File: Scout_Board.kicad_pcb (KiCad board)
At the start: 2 copper layers, 102.5 x 80 mm, 57 parts, among them J1 Conn_01x01_Pin, J2 Conn_01x04_Pin, J3 RAPC722X, J4 Screw_Terminal_01x02, J5 5V, J6 GND, Q1 BSS138, Q2 BSS138, U1 DRV8871DDA, U2 ESP32-S3-DEVKITC-1U-N8R2, U3 LM2576HVS-5, U4 LM2576HVS-5

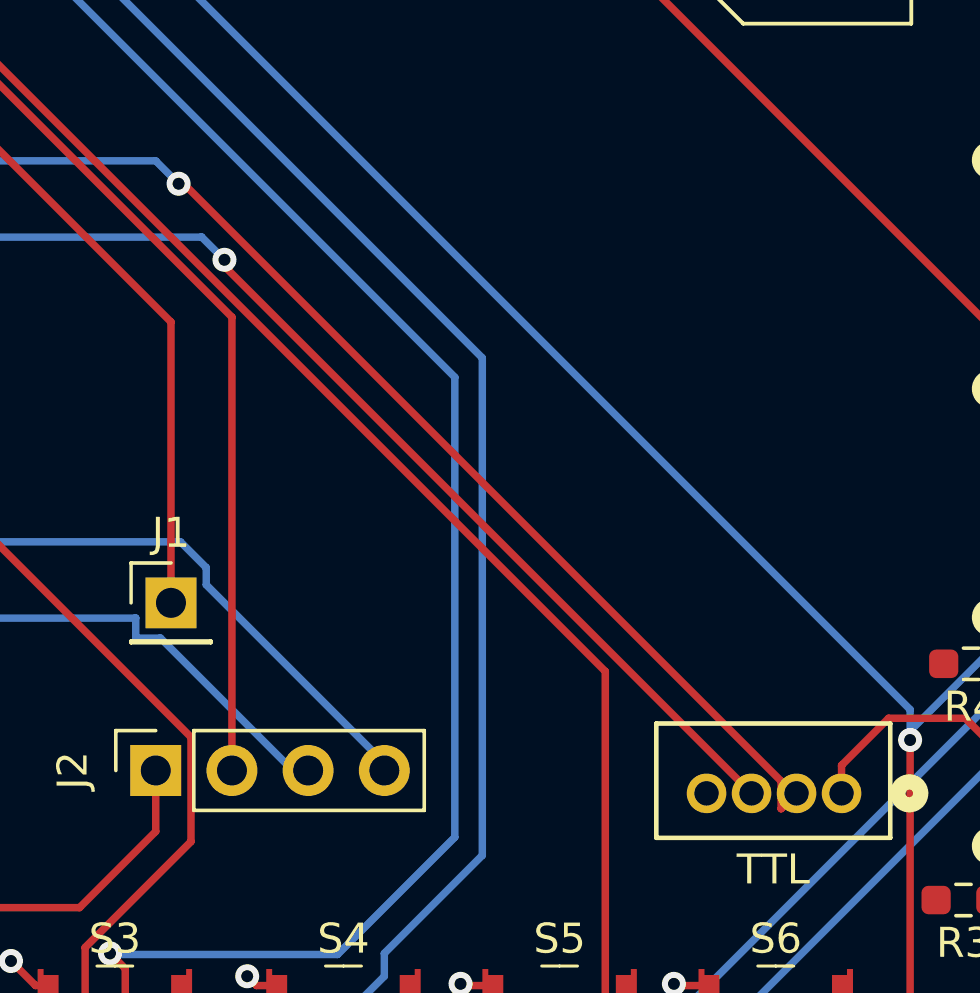
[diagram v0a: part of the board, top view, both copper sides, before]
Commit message: New Branch - Alpha2.0
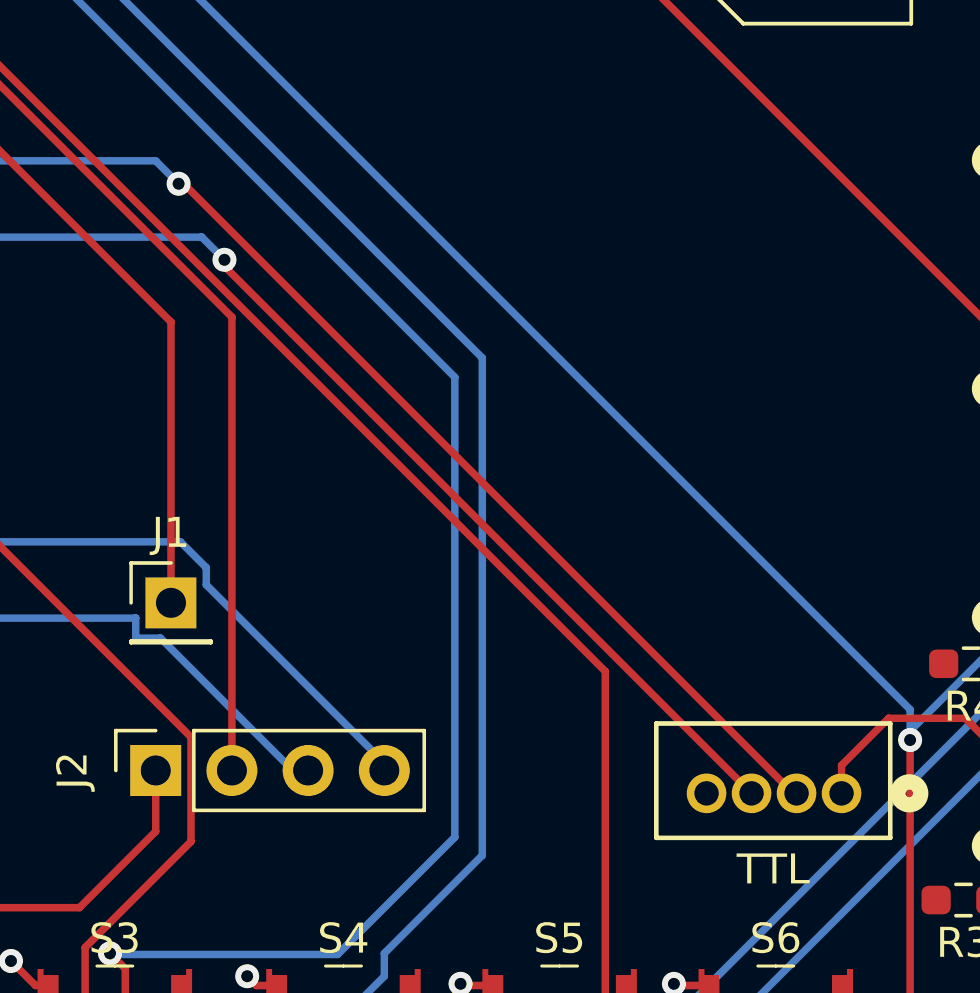
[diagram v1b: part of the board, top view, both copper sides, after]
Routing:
- net RxD: track 41.0 -> 40.0 mm
